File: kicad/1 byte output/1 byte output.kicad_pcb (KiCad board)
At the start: 2 copper layers, 52.1 x 53.3 mm, 9 parts, among them J1 Conn_01x05_Male, J2 Conn_01x05_Female, J3 Conn_01x08, J4 Screw_Terminal_01x02, U1 74HCT595, U2 ULN2803A

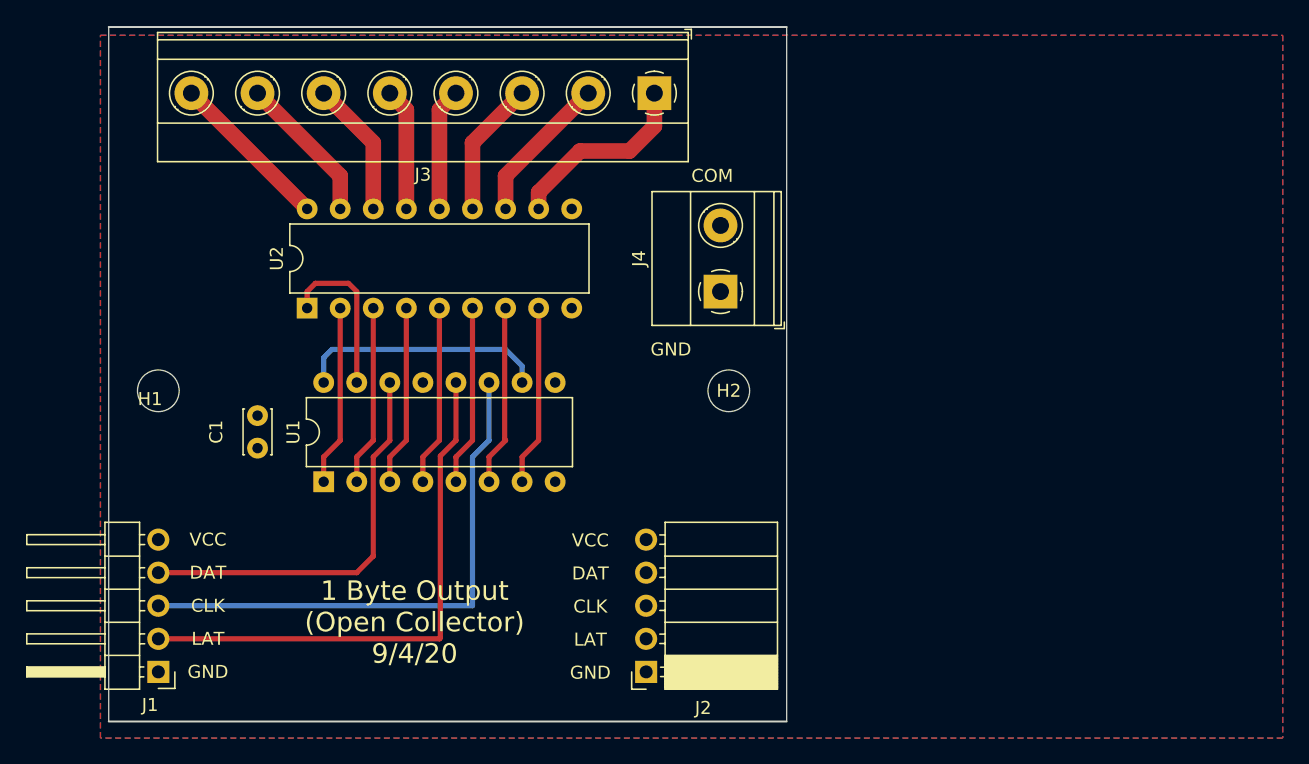
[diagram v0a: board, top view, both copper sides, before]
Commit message: periodic check in
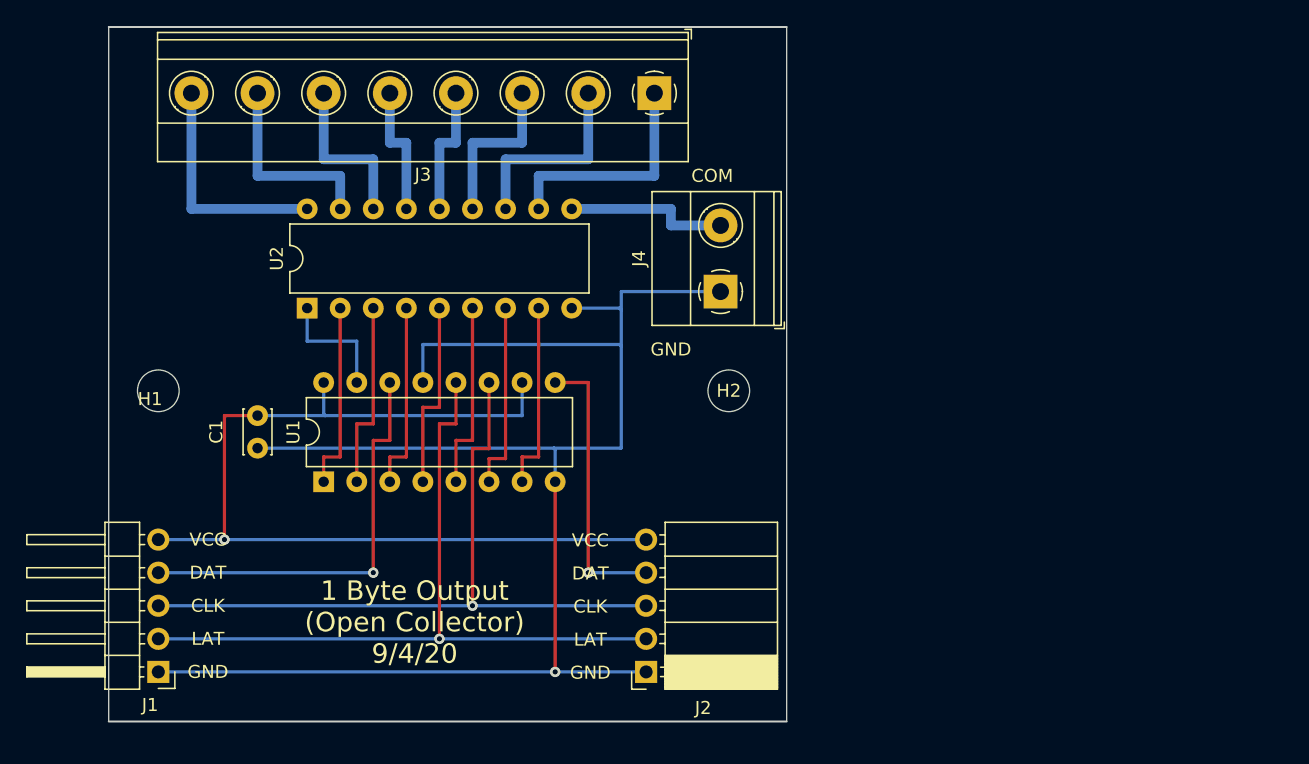
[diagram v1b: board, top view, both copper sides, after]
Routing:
- net GND: track 0.00 -> 124.3 mm, vias 0 -> 1
- net VCC: track 19.2 -> 75.0 mm, vias 0 -> 2
- net DO: track 0.00 -> 21.6 mm, vias 0 -> 1
- net LAT: track 41.8 -> 58.4 mm, vias 0 -> 1
- net CLK: track 41.8 -> 55.9 mm, vias 0 -> 1
- net COM: track 0.00 -> 12.7 mm
- net OUT1: track 12.6 -> 17.8 mm
- net OUT2: track 11.5 -> 15.2 mm
- net OUT7: track 11.5 -> 15.2 mm
- net Net-(U1-Pad15): track 12.6 -> 9.52 mm
- net OUT8: track 14.8 -> 17.8 mm
- net OUT3: track 10.5 -> 12.7 mm
- net OUT6: track 10.5 -> 12.7 mm
- net DI: track 30.9 -> 32.4 mm, vias 0 -> 1
- net OUT5: track 9.42 -> 10.2 mm
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- removed copper zone on B.Cu, net GND
- removed copper zone on F.Cu, net VCC
